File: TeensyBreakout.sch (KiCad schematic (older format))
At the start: 56 parts, among them IC1 ZLDO1117G33, IC2 NCP1117ST50T3G, J1 73725-0110BLF, J3 RJ45_LED, J4 PJ-102A, Q1 FDN340P, Q1A1 BSD223P, Q1B1 BSD223P, SW1 SW_MEC_5E, U1 Teensy4.1, U2 ESP-WROOM-02

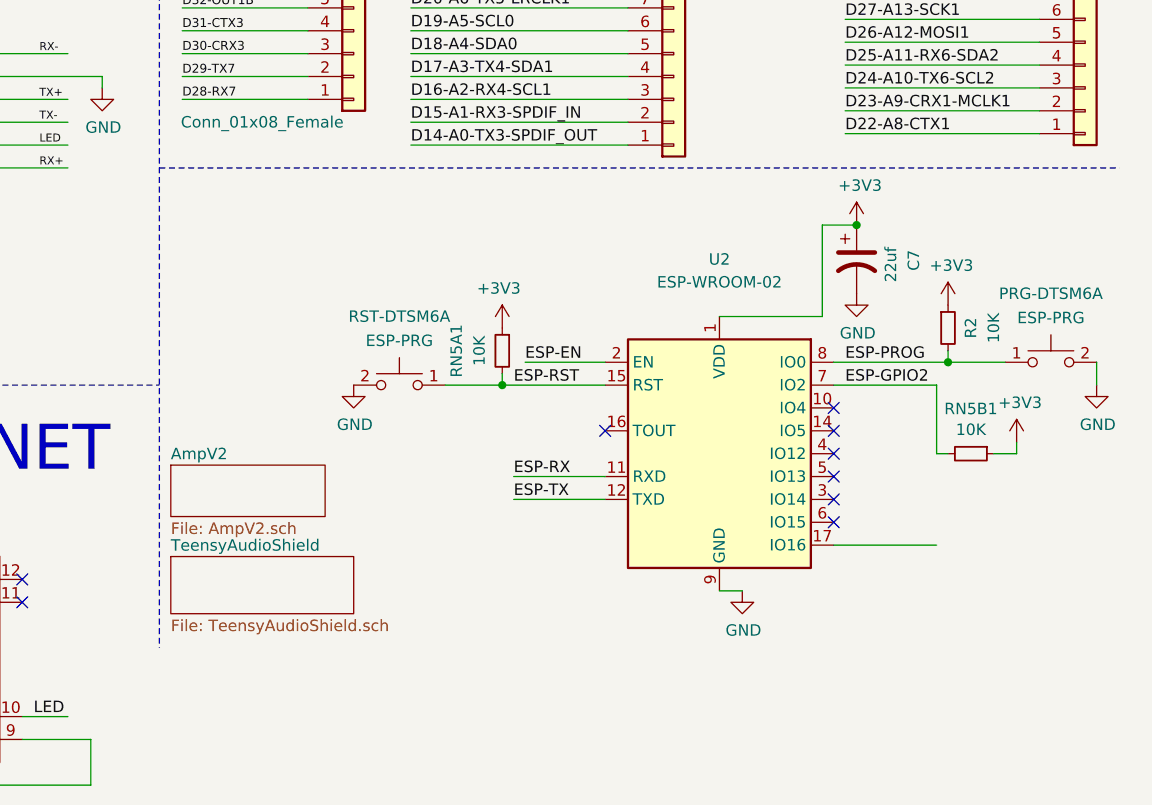
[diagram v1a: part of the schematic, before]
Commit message: gonna try auto-route
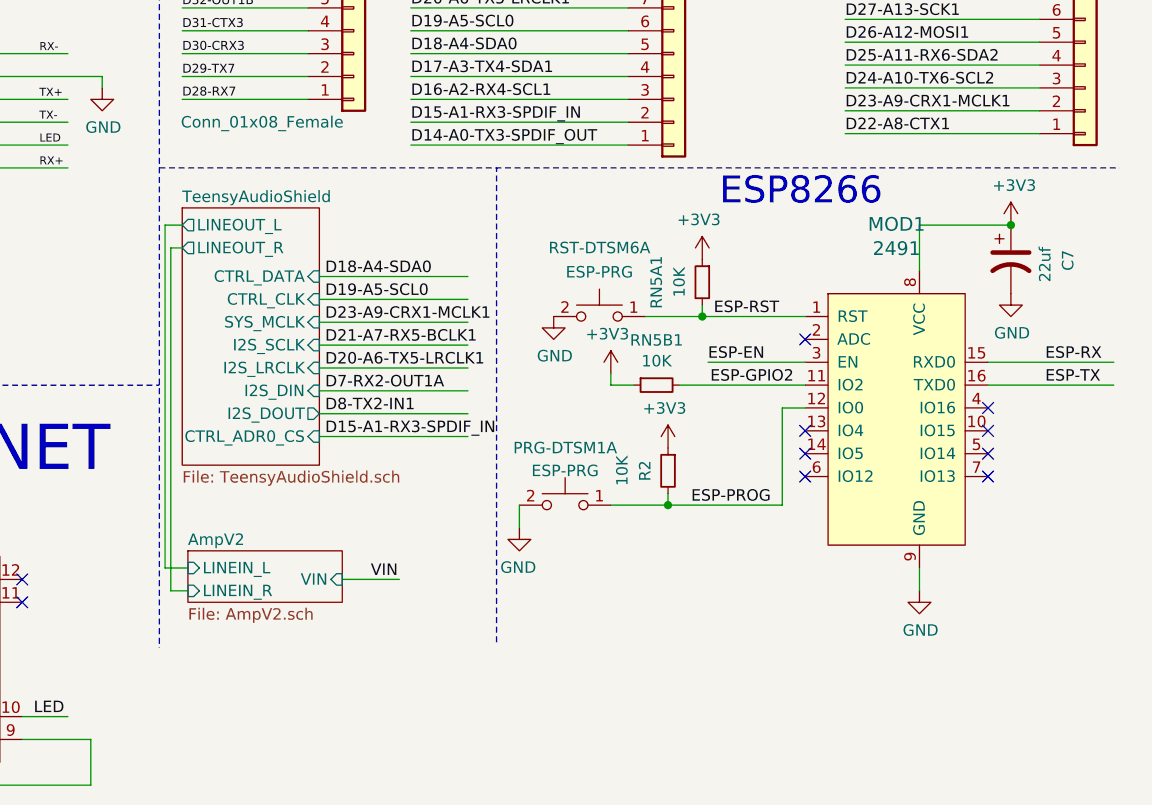
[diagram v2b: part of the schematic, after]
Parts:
- removed PRG-DTSM6: ESP-PRG, Button_Switch_THT:SW_PUSH_6mm, symbol Switch:SW_Push_Dual_x2
- removed U2: ESP-WROOM-02, RF_Module:ESP-WROOM-02, symbol RF_Module:ESP-WROOM-02
- added MOD1: 2491, digikey-footprints:WIFI_Module_ESP8266_2491, symbol dk_RF-Transceiver-Modules:2491
- added PRG-DTSM1: ESP-PRG, Button_Switch_THT:SW_PUSH_6mm, symbol Switch:SW_Push_Dual_x2
- SPI1: footprint Connector_PinSocket_2.54mm:PinSocket_2x03_P2.54mm_Vertical -> CustomFootprints:PinSocket_2x03_P2.54mm_Vertical(Flipped)
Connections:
- wire segments 274 -> 287
- no-connect marks 17 -> 18
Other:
- note added: "ESP8266"
- moved on the sheet: RN5A1, RST-DTSM6A
